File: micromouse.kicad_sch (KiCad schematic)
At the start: 15 parts, among them J1 XT60-M, SW1 SW_SPST, SW2 SW_Push, SW3 SW_SPDT_312, SW4 SW_Push, U1 BUCK, U2 STM32 Blackpill, U3 N20 encoder right, U4 N20 encoder left, U5 TB6612FNG, U6 VL53L0X left, U7 VL53L0X right, U8 VL53L0X middle, U9 oled i2c

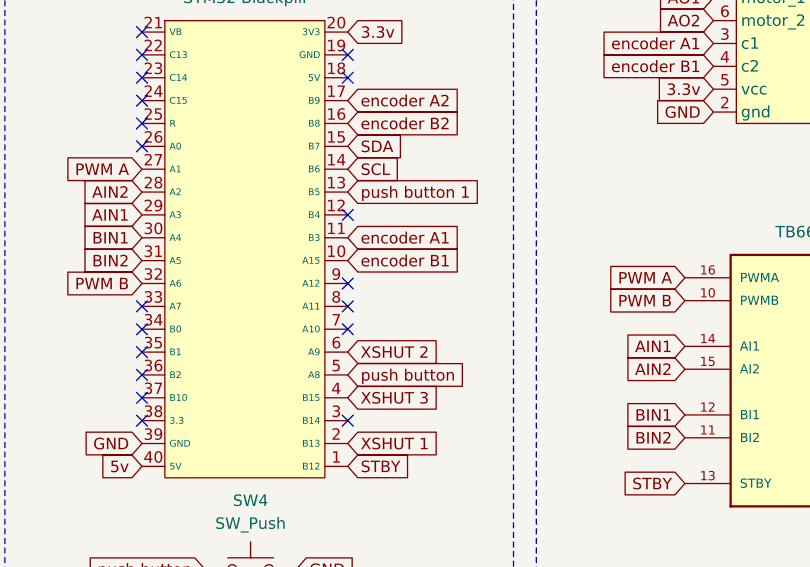
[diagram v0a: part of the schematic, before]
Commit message: ch
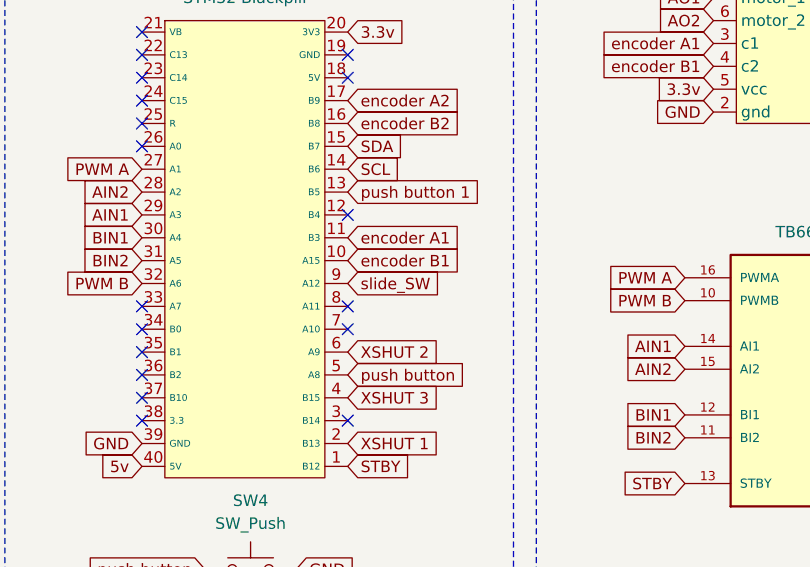
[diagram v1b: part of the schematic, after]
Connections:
- net slide_SW: now also U2.9 (A12)
- no-connect marks 26 -> 25
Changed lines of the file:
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@@
-	)
-	(no_connect
-		(at 90.17 77.47)
 	)
 	(no_connect
@@
 				(hide yes)
 			)
+		)
+	)
+	(global_label "slide_SW"
+		(shape input)
+		(at 90.17 77.47 0)
+		(fields_autoplaced yes)
+		(effects
+			(font
+				(size 1.27 1.27)
+			)
+			(justify left)
+		)
+		(property "Intersheetrefs" "${INTERSHEET_REFS}"
+			(at 101.3194 77.47 0)
+			(effects
+				(font
+					(size 1.27 1.27)
+				)
+				(justify left)
+				(hide yes)
+			)

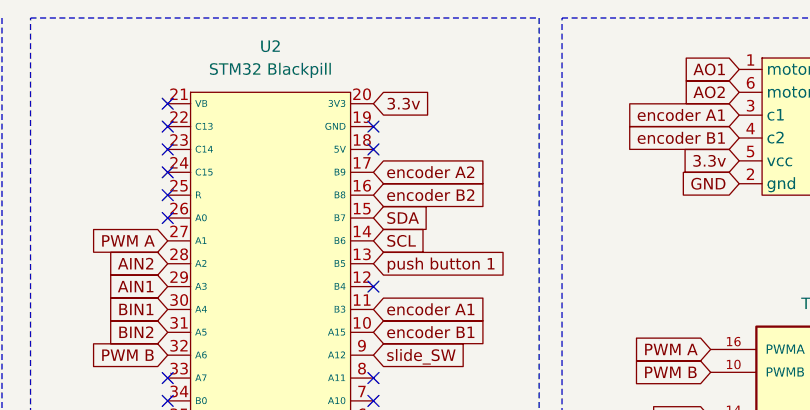
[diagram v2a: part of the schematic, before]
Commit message: pcb changes!!!!!
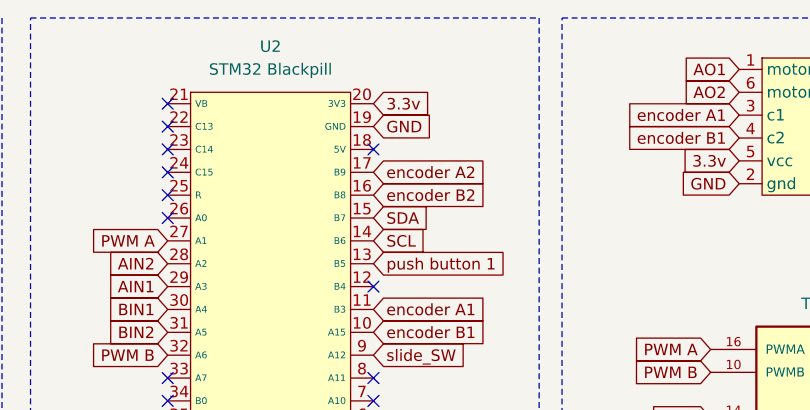
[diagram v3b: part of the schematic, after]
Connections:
- net GND: now also U2.19 (GND)
- no-connect marks 25 -> 24
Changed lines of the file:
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@@
-	)
-	(no_connect
-		(at 90.17 52.07)
 	)
 	(no_connect
@@
 			(effects
 				(font
+					(size 1.27 1.27)
+				)
+				(justify left)
+				(hide yes)
+			)
+		)
+	)
+	(global_label "GND"
+		(shape input)
+		(at 90.17 52.07 0)
+		(fields_autoplaced yes)
+		(effects
+			(font
+				(size 1.27 1.27)
+			)
+			(justify left)
+		)
+		(property "Intersheetrefs" "${INTERSHEET_REFS}"
+			(at 97.0257 52.07 0)
+			(effects
+				(font

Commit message: pcb
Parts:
- SW2, SW4: footprint push button:push_button -> push button 1:SW_VS-1213-67-160GF
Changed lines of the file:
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@@
 			)
 		)
-		(property "Footprint" "push button:push_button"
+		(property "Footprint" "push button 1:SW_VS-1213-67-160GF"
 			(at 78.74 116.205 0)
 			(effects
@@
 			)
 		)
-		(property "Footprint" "push button:push_button"
+		(property "Footprint" "push button 1:SW_VS-1213-67-160GF"
 			(at 79.375 104.14 0)
 			(effects

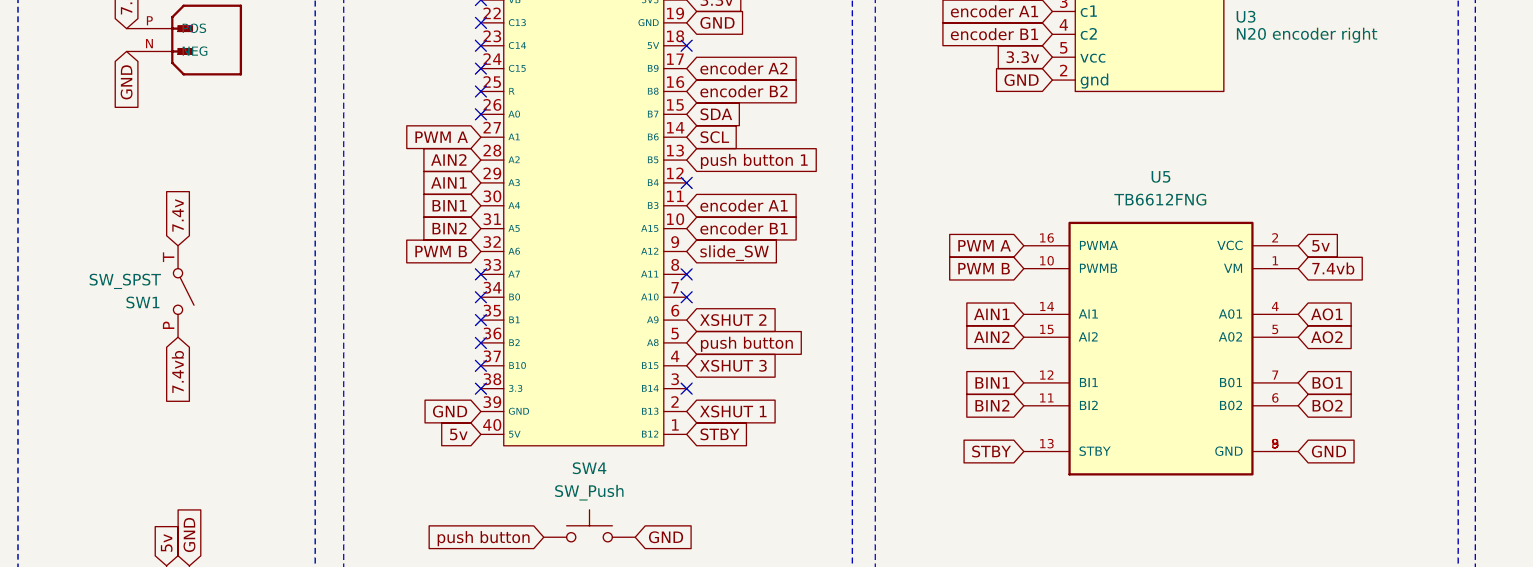
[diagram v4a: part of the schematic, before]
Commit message: pcb
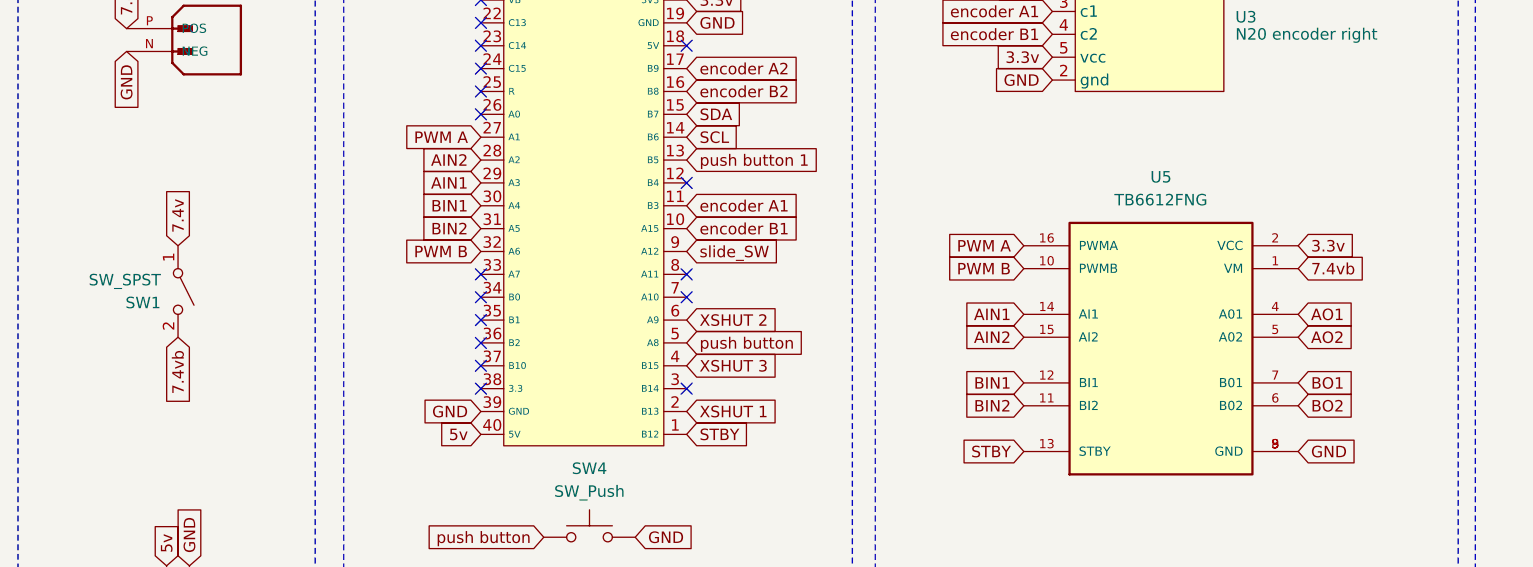
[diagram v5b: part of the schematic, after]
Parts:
- SW1: footprint SPST:JUDCOSPST -> power switch:battery_sw
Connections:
- net 3.3v: now also U5.2 (VCC)
- net 5v: no longer U5.2 (VCC)
- net 7.4v: now also SW1.1 (A); no longer SW1.T (A)
- net 7.4vb: now also SW1.2 (B); no longer SW1.P (B)
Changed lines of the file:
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@@
 		)
 	)
-	(global_label "5v"
+	(global_label "3.3v"
 		(shape input)
 		(at 158.115 76.835 0)
@@
 		)
 		(property "Intersheetrefs" "${INTERSHEET_REFS}"
-			(at 163.2773 76.835 0)
+			(at 165.0916 76.835 0)
 			(effects
 				(font
@@
 			)
 		)
-		(property "Footprint" "SPST:JUDCOSPST"
+		(property "Footprint" "power switch:battery_sw"
 			(at 33.655 81.915 0)
 			(effects
@@
 			)
 		)
-		(pin "T"
+		(pin "2"
 		)
-		(pin "P"
+		(pin "1"
 		)
 		(instances

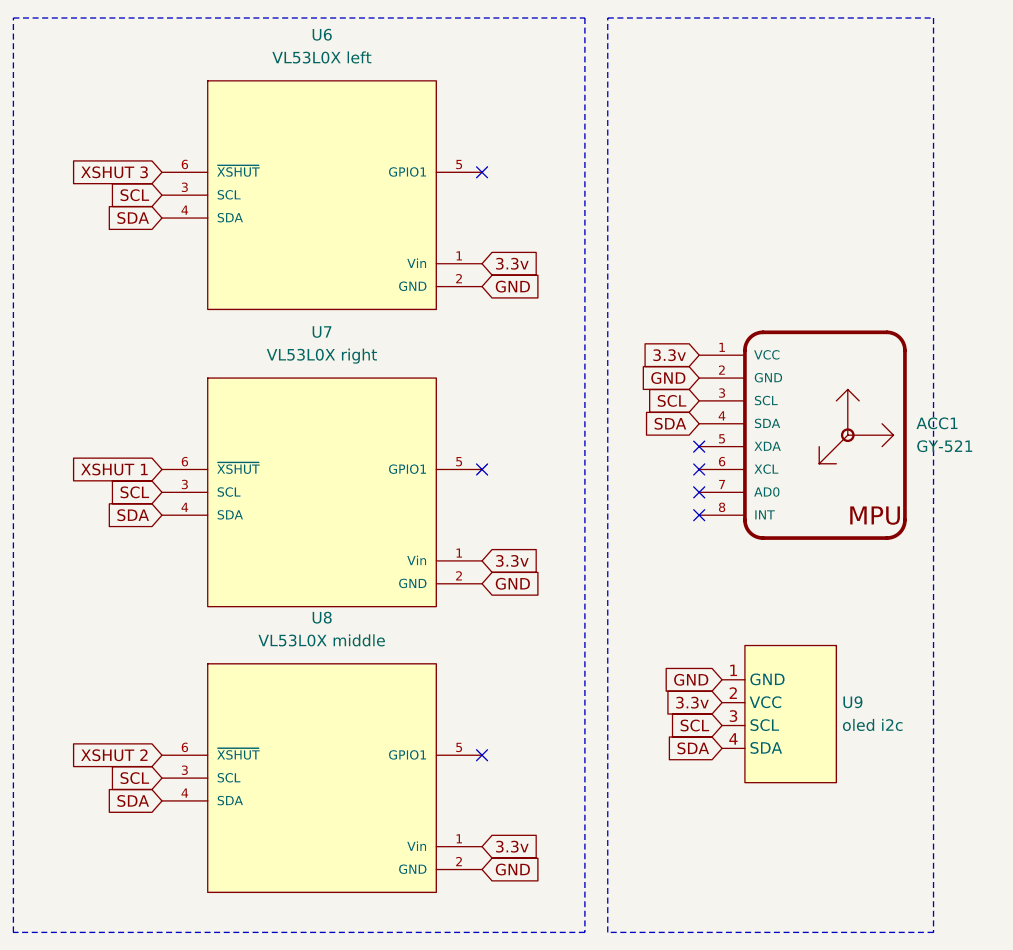
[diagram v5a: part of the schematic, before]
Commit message: hello world
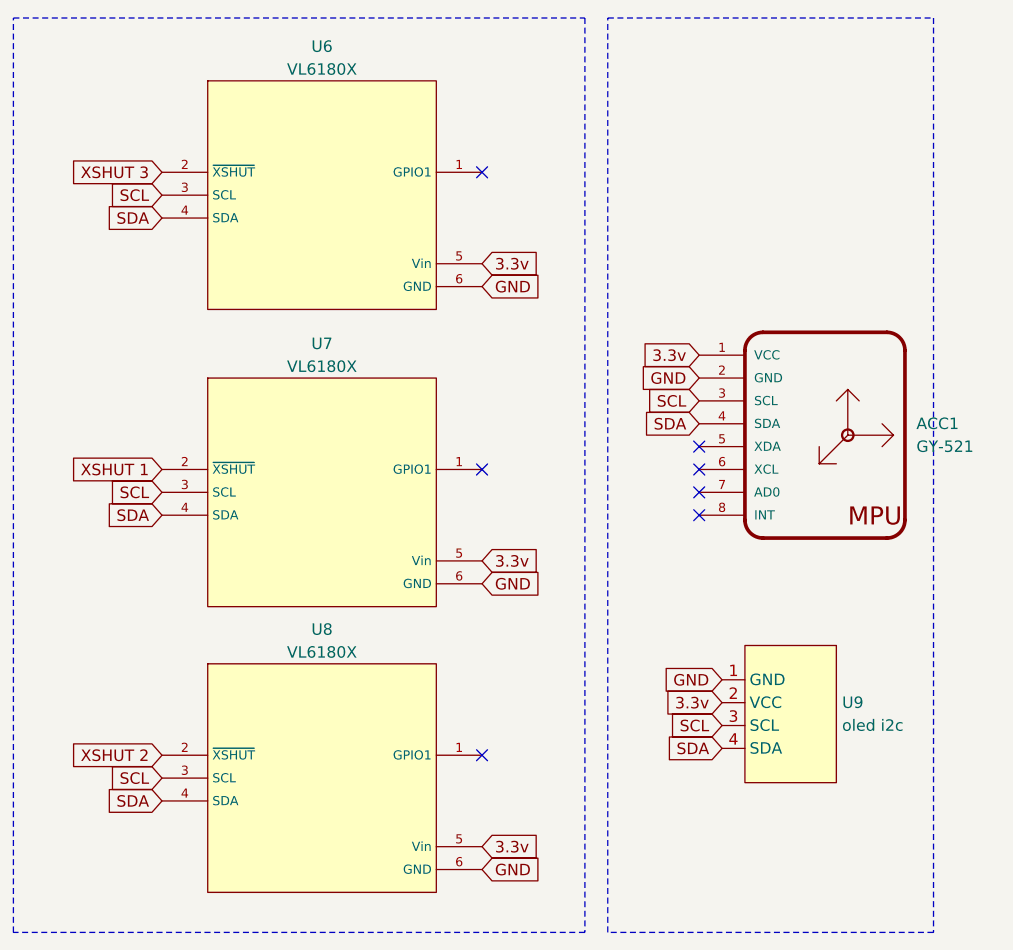
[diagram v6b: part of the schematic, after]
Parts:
- removed U6: VL53L0X left, VL53L0X:VL53L0X, symbol VL53L0X:VL53L0X
- removed U7: VL53L0X right, VL53L0X:VL53L0X, symbol VL53L0X:VL53L0X
- removed U8: VL53L0X middle, VL53L0X:VL53L0X, symbol VL53L0X:VL53L0X
- added U6, U7, U8: VL6180X, VL6180X:VL6180X, symbol VL53L0X:VL6180x
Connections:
- net 3.3v: now also U6.5 (Vin), U7.5 (Vin), U8.5 (Vin)
- net GND: now also U6.6 (GND), U7.6 (GND), U8.6 (GND)
- net SCL: now also U6.3 (SCL), U7.3 (SCL), U8.3 (SCL)
- net SDA: now also U6.4 (SDA), U7.4 (SDA), U8.4 (SDA)
- net XSHUT 1: now also U7.2 (~{XSHUT})
- net XSHUT 2: now also U8.2 (~{XSHUT})
- net XSHUT 3: now also U6.2 (~{XSHUT})
